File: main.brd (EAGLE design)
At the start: 24.4 x 26.2 mm, 36 parts, among them IC1 ATTINY13A-SSH, IC2 TP4056-42-ESOP8, IC3 LM27313XMFX_NOPB, T1A 2N4401, T1B NPN, X1 MINI-USB-UX60A-MB-5ST, X2 332-02

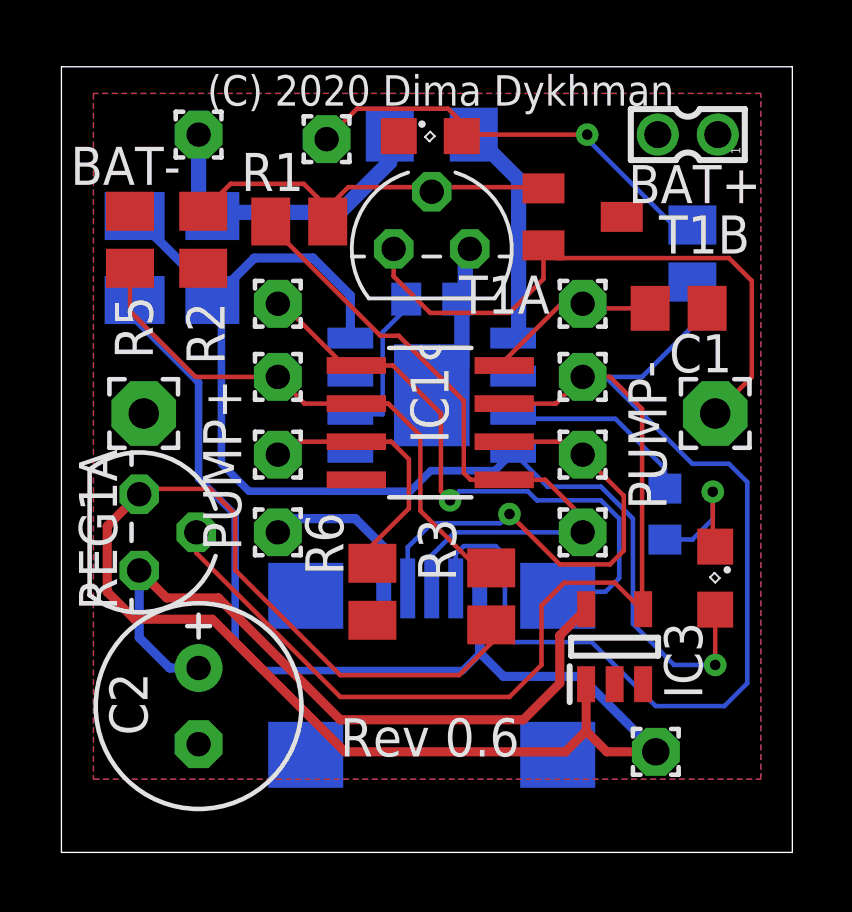
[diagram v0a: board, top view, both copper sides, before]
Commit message: improved solar
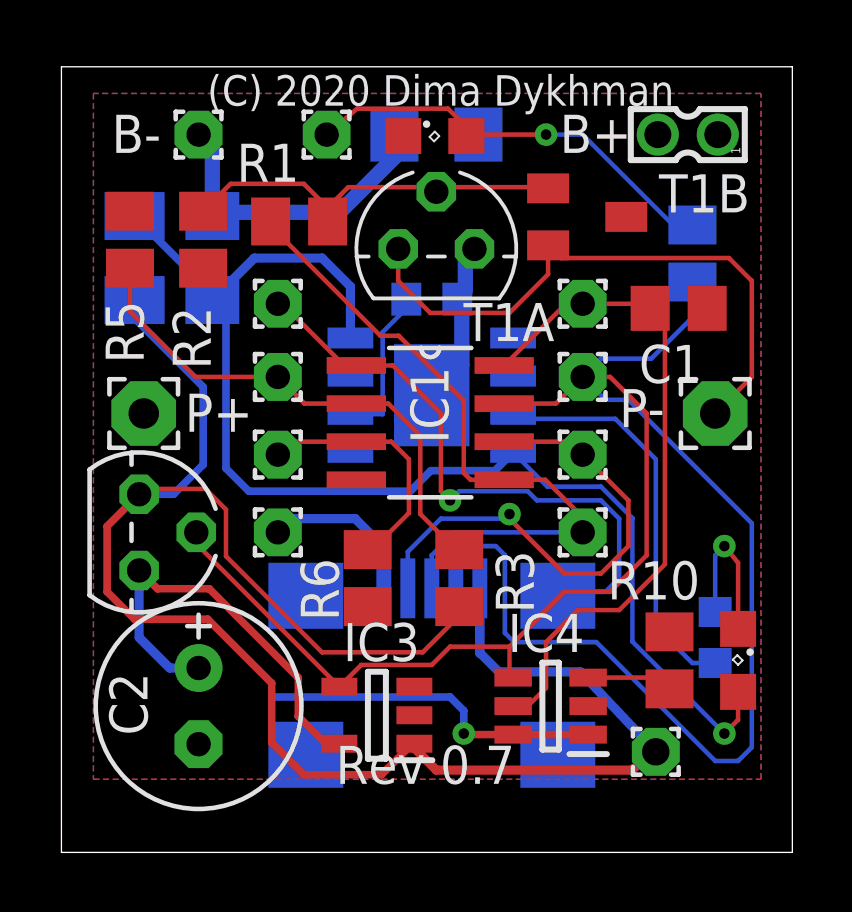
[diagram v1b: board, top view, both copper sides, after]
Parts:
- added IC4: TPL5110DDCT, SamacSys:SOT95P280X110-6N
- added R10: 100k, resistor:M0805
- moved IC3 8.25 mm to (11.4, 3.66), turned to 180 degrees
- moved R8 4.44 mm to (22.7, 6.25), turned to 270 degrees
- moved LED2 2.85 mm to (23.5, 5.49)
- moved R3 1.23 mm to (14.2, 8.23)
- moved R6 0.48 mm to (11.1, 8.23)
- moved LED1 0.15 mm to (13.4, 23.0)
- moved PAD1 0.15 mm to (9.75, 23.0)
- moved T1B 0.15 mm to (18.4, 20.3)
- moved C4 0.15 mm to (13.4, 23.0)
- moved T1A 0.15 mm to (13.4, 19.2)
- turned C1 to 180 degrees
- turned IN+ to 90 degrees
- renumbered BAT- to B-
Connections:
- new net N$3: C1.2, IC1.8, IC4.5, PAD3.1
- new net N$7: IC4.3, R10.1
- net GND: now also C1.1, IC4.2, R10.2; no longer C1.2
- net SOLAR: now also IC4.4
- net VCC: now also IC4.1, IC4.6; no longer C1.1, IC1.8, PAD3.1
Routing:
- net N$3: track 0.00 -> 22.4 mm
- net N$5: track 76.0 -> 62.0 mm
- net SOLAR_PANEL+: track 24.1 -> 14.5 mm
- net N$8: track 6.48 -> 13.4 mm
- net N$7: track 0.00 -> 2.87 mm
- net VCC: track 13.3 -> 11.5 mm, vias 0 -> 1
- net N$4: track 40.8 -> 42.3 mm
- net UART_TX: track 18.5 -> 17.2 mm
- net N$9: track 4.65 -> 5.25 mm
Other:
- board text added: "B+"
- board text added: "B-"
- board text added: "P+"
- board text added: "P-"
- board text added: "Rev 0.7"
- board text removed: "BAT+"
- board text removed: "BAT-"
- board text removed: "Rev 0.6"
